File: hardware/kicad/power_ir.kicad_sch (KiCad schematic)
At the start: 0 parts

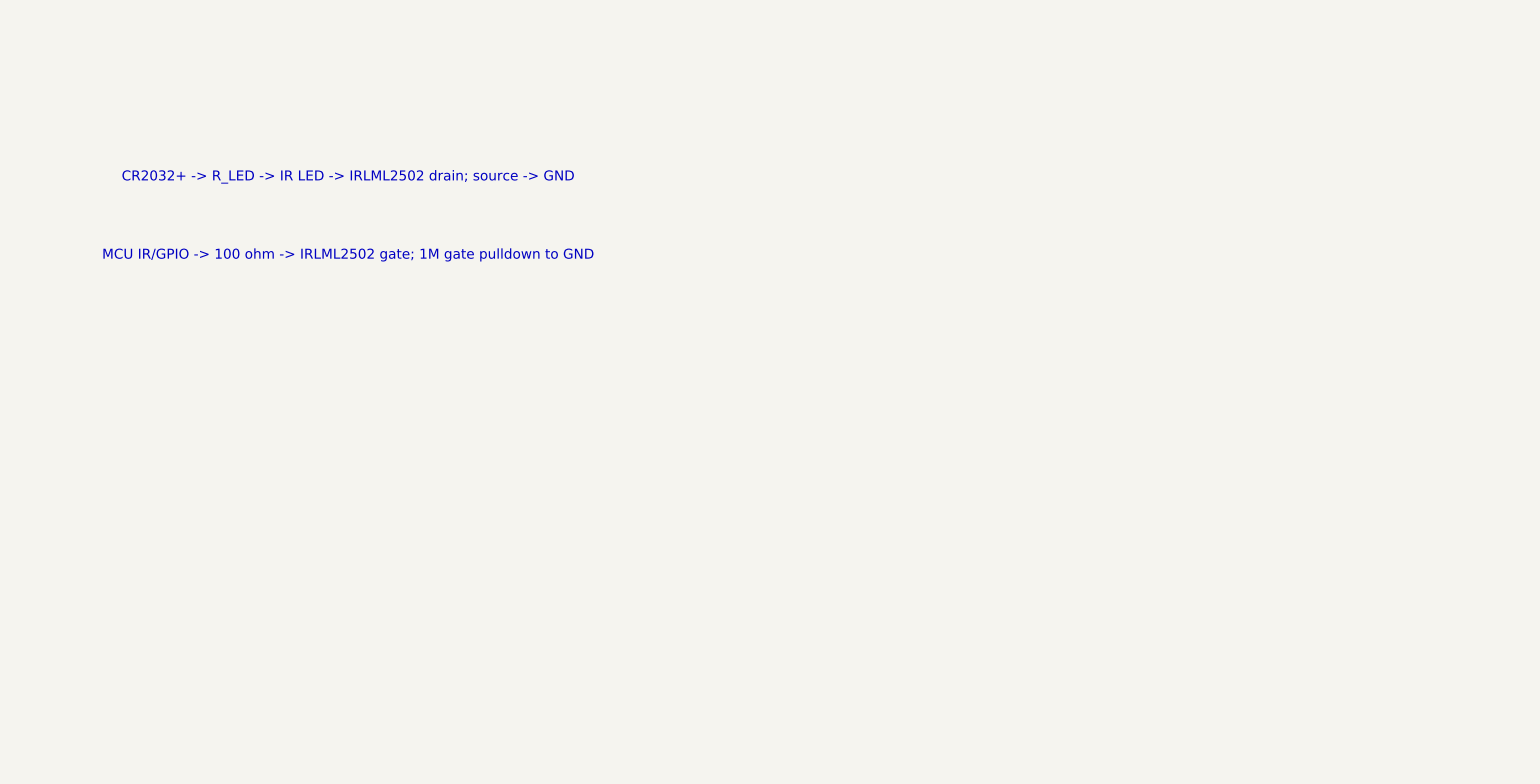
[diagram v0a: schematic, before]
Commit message: sch opt
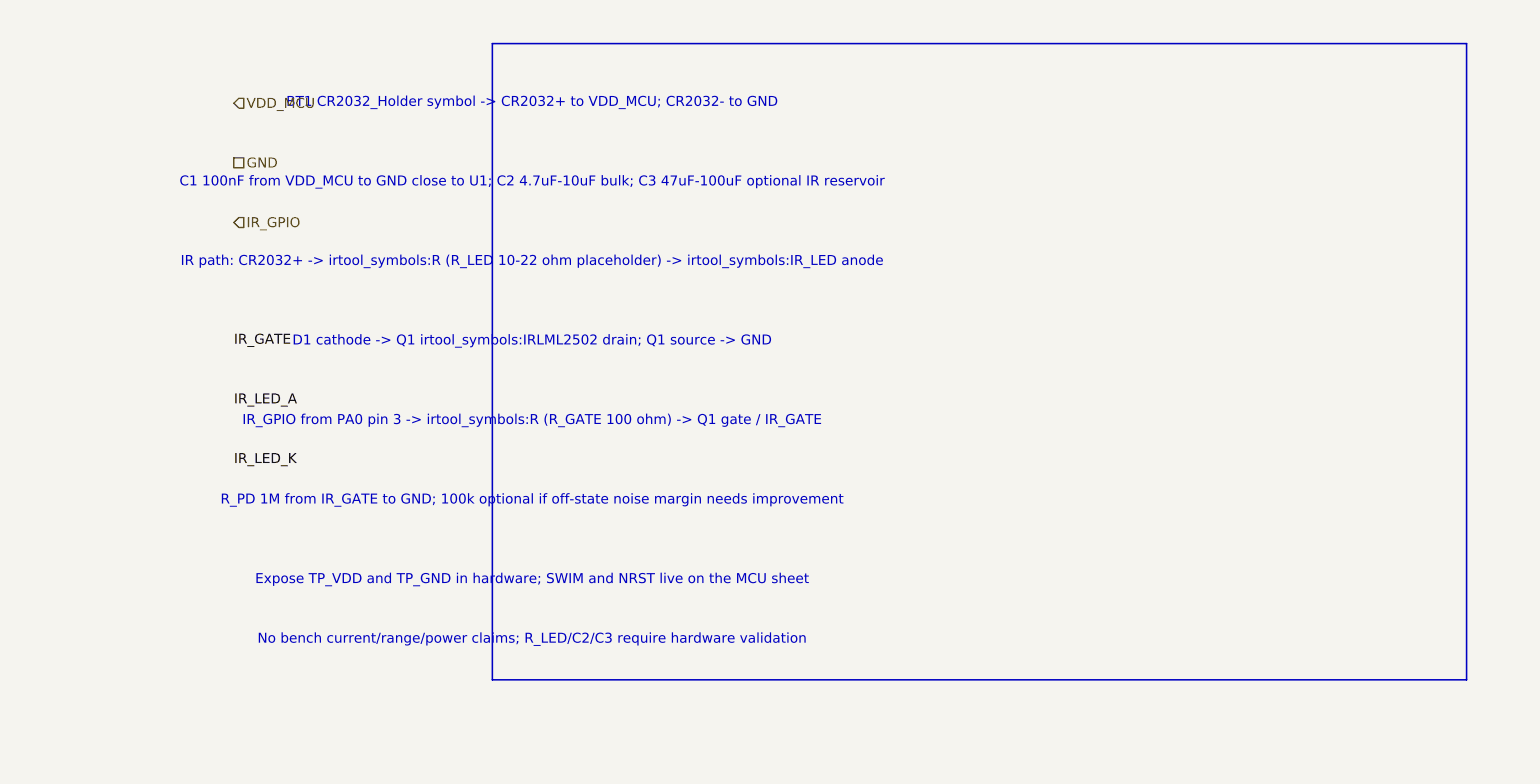
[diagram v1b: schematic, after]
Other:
- note added: "BT1 CR2032_Holder symbol -> CR2032+ to VDD_MCU; CR2032- to GND"
- note added: "C1 100nF from VDD_MCU to GND close to U1; C2 4.7uF-10uF bulk; C3 47uF-100uF optional IR reservoir"
- note added: "D1 cathode -> Q1 irtool_symbols:IRLML2502 drain; Q1 source -> GND"
- note added: "Expose TP_VDD and TP_GND in hardware; SWIM and NRST live on the MCU sheet"
- note added: "IR path: CR2032+ -> irtool_symbols:R (R_LED 10-22 ohm placeholder) -> irtool_symbols:IR_LED anode"
- note added: "IR_GPIO from PA0 pin 3 -> irtool_symbols:R (R_GATE 100 ohm) -> Q1 gate / IR_GATE"
- note added: "No bench current/range/power claims; R_LED/C2/C3 require hardware validation"
- note added: "R_PD 1M from IR_GATE to GND; 100k optional if off-state noise margin needs improvement"
- note removed: "CR2032+ -> R_LED -> IR LED -> IRLML2502 drain; source -> GND"
- note removed: "MCU IR/GPIO -> 100 ohm -> IRLML2502 gate; 1M gate pulldown to GND"
- title: Power and IR Driver Skeleton -> Power and IR Driver - Electrical Skeleton
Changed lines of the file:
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@@
 (kicad_sch (version 20230121) (generator "codex")
   (paper "A4")
-  (title_block (title "Power and IR Driver Skeleton"))
-  (text "CR2032+ -> R_LED -> IR LED -> IRLML2502 drain; source -> GND" (at 40 40 0) (effects (font (size 1.27 1.27))))
-  (text "MCU IR/GPIO -> 100 ohm -> IRLML2502 gate; 1M gate pulldown to GND" (at 40 50 0) (effects (font (size 1.27 1.27))))
+  (title_block (title "Power and IR Driver - Electrical Skeleton"))
+  (hierarchical_label "VDD_MCU" (shape input) (at 25.4 30.48 0)
+    (effects (font (size 1.27 1.27)))
+  )
+  (hierarchical_label "GND" (shape passive) (at 25.4 38.1 0)
+    (effects (font (size 1.27 1.27)))
+  )
+  (hierarchical_label "IR_GPIO" (shape input) (at 25.4 45.72 0)
+    (effects (font (size 1.27 1.27)))
+  )
+  (label "IR_GATE" (at 25.4 60.96 0)
+    (effects (font (size 1.27 1.27)))
+  )
+  (label "IR_LED_A" (at 25.4 68.58 0)
+    (effects (font (size 1.27 1.27)))
+  )
+  (label "IR_LED_K" (at 25.4 76.2 0)
+    (effects (font (size 1.27 1.27)))
+  )
+  (polyline
+    (pts (xy 58.42 22.86) (xy 182.88 22.86) (xy 182.88 104.14) (xy 58.42 104.14) (xy 58.42 22.86))
+    (stroke (width 0.2) (type default) (color 0 0 0 0))
+  )
+  (text "BT1 CR2032_Holder symbol -> CR2032+ to VDD_MCU; CR2032- to GND" (at 63.5 30.48 0)
+    (effects (font (size 1.27 1.27)))
+  )
+  (text "C1 100nF from VDD_MCU to GND close to U1; C2 4.7uF-10uF bulk; C3 47uF-100uF optional IR reservoir" (at 63.5 40.64 0)
+    (effects (font (size 1.27 1.27)))
+  )
+  (text "IR path: CR2032+ -> irtool_symbols:R (R_LED 10-22 ohm placeholder) -> irtool_symbols:IR_LED anode" (at 63.5 50.8 0)
+    (effects (font (size 1.27 1.27)))
+  )
+  (text "D1 cathode -> Q1 irtool_symbols:IRLML2502 drain; Q1 source -> GND" (at 63.5 60.96 0)
+    (effects (font (size 1.27 1.27)))
+  )
+  (text "IR_GPIO from PA0 pin 3 -> irtool_symbols:R (R_GATE 100 ohm) -> Q1 gate / IR_GATE" (at 63.5 71.12 0)
+    (effects (font (size 1.27 1.27)))
+  )
+  (text "R_PD 1M from IR_GATE to GND; 100k optional if off-state noise margin needs improvement" (at 63.5 81.28 0)
+    (effects (font (size 1.27 1.27)))
+  )
+  (text "Expose TP_VDD and TP_GND in hardware; SWIM and NRST live on the MCU sheet" (at 63.5 91.44 0)
+    (effects (font (size 1.27 1.27)))
+  )
+  (text "No bench current/range/power claims; R_LED/C2/C3 require hardware validation" (at 63.5 99.06 0)
+    (effects (font (size 1.27 1.27)))
+  )
+  (path "/" (page "3"))
 )

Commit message: add pcb
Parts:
- added BT1: CR2032
- added C1: 100n
- added D1: 940nm
- added Q1: IRLML2502
- added R1: R_LED
- added R2: R_GATE
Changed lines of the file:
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@@
     (stroke (width 0.2) (type default) (color 0 0 0 0))
+  )
+  (symbol "irtool_symbols:CR2032_Holder" (at 88.9 35.56 0) (unit 1) (in_bom yes) (on_board yes)
+    (property "Reference" "BT1" (at 88.9 30.48 0) (effects (font (size 1.27 1.27))))
+    (property "Value" "CR2032" (at 88.9 40.64 0) (effects (font (size 1.27 1.27))))
+    (pin "1")
+    (pin "2")
+    (instances (project "remote" (path "/d90b45e5-8bd2-48de-af1a-b95d5a3f3001" (reference "BT1") (unit 1))))
+  )
+  (symbol "irtool_symbols:R" (at 119.38 50.8 0) (unit 1) (in_bom yes) (on_board yes)
+    (property "Reference" "R1" (at 119.38 48.26 0) (effects (font (size 1.27 1.27))))
+    (property "Value" "R_LED" (at 119.38 53.34 0) (effects (font (size 1.27 1.27))))
+    (pin "1")
+    (pin "2")
+    (instances (project "remote" (path "/d90b45e5-8bd2-48de-af1a-b95d5a3f3001" (reference "R1") (unit 1))))
+  )
+  (symbol "irtool_symbols:IR_LED" (at 149.86 50.8 0) (unit 1) (in_bom yes) (on_board yes)
+    (property "Reference" "D1" (at 149.86 46.99 0) (effects (font (size 1.27 1.27))))
+    (property "Value" "940nm" (at 149.86 54.61 0) (effects (font (size 1.27 1.27))))
+    (pin "1")
+    (pin "2")
+    (instances (project "remote" (path "/d90b45e5-8bd2-48de-af1a-b95d5a3f3001" (reference "D1") (unit 1))))
+  )
+  (symbol "irtool_symbols:IRLML2502" (at 149.86 71.12 0) (unit 1) (in_bom yes) (on_board yes)
+    (property "Reference" "Q1" (at 149.86 66.04 0) (effects (font (size 1.27 1.27))))
+    (property "Value" "IRLML2502" (at 149.86 76.2 0) (effects (font (size 1.27 1.27))))
+    (pin "1")
+    (pin "2")
+    (pin "3")
+    (instances (project "remote" (path "/d90b45e5-8bd2-48de-af1a-b95d5a3f3001" (reference "Q1") (unit 1))))
+  )
+  (symbol "irtool_symbols:R" (at 119.38 71.12 0) (unit 1) (in_bom yes) (on_board yes)
+    (property "Reference" "R2" (at 119.38 68.58 0) (effects (font (size 1.27 1.27))))
+    (property "Value" "R_GATE" (at 119.38 73.66 0) (effects (font (size 1.27 1.27))))
+    (pin "1")
+    (pin "2")
+    (instances (project "remote" (path "/d90b45e5-8bd2-48de-af1a-b95d5a3f3001" (reference "R2") (unit 1))))
+  )
+  (symbol "irtool_symbols:C" (at 88.9 55.88 0) (unit 1) (in_bom yes) (on_board yes)
+    (property "Reference" "C1" (at 88.9 53.34 0) (effects (font (size 1.27 1.27))))
+    (property "Value" "100n" (at 88.9 58.42 0) (effects (font (size 1.27 1.27))))
+    (pin "1")
+    (pin "2")
+    (instances (project "remote" (path "/d90b45e5-8bd2-48de-af1a-b95d5a3f3001" (reference "C1") (unit 1))))
   )
   (text "BT1 CR2032_Holder symbol -> CR2032+ to VDD_MCU; CR2032- to GND" (at 63.5 30.48 0)

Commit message: pcb opt
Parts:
- removed C1: 100n
- added BT1: CR2032
- added C2: 4.7uF
- added C3: 47u..100u OPT
- added R_PD: 1M
- C1: renamed from BT1; value CR2032 -> 100nF
- D1: value 940nm -> 940nm IR
- R1: value R_LED -> 10-22R
- R2: value R_GATE -> 100R
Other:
- note added: "C1/C2 mandatory decoupling; C3 optional IR burst reservoir (47-100uF, validate leakage)"
- note added: "IRLML2502 low-side topology: G=R2/IR_GATE, D=IR_LED_K, S=GND"
- note added: "R1 limits IR LED current from CR2032+. Final 10-22R value requires bench validation."
- note removed: "BT1 CR2032_Holder symbol -> CR2032+ to VDD_MCU; CR2032- to GND"
- note removed: "C1 100nF from VDD_MCU to GND close to U1; C2 4.7uF-10uF bulk; C3 47uF-100uF optional IR reservoir"
- note removed: "D1 cathode -> Q1 irtool_symbols:IRLML2502 drain; Q1 source -> GND"
- note removed: "Expose TP_VDD and TP_GND in hardware; SWIM and NRST live on the MCU sheet"
- note removed: "IR path: CR2032+ -> irtool_symbols:R (R_LED 10-22 ohm placeholder) -> irtool_symbols:IR_LED anode"
- note removed: "IR_GPIO from PA0 pin 3 -> irtool_symbols:R (R_GATE 100 ohm) -> Q1 gate / IR_GATE"
- note removed: "No bench current/range/power claims; R_LED/C2/C3 require hardware validation"
- note removed: "R_PD 1M from IR_GATE to GND; 100k optional if off-state noise margin needs improvement"
- title: Power and IR Driver - Electrical Skeleton -> Power and IR Driver
